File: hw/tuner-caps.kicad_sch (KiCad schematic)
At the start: 30 parts, among them K2101 G2RL-2, K2102 G2RL-2, K2103 G2RL-2, K2104 G2RL-2, K2105 G2RL-2, K2106 G2RL-2, K2107 G2RL-2, K2108 G2RL-2, K2109 G2RL-2, U2101 TPIC6C595PWR, U2102 TPIC6C595PWR

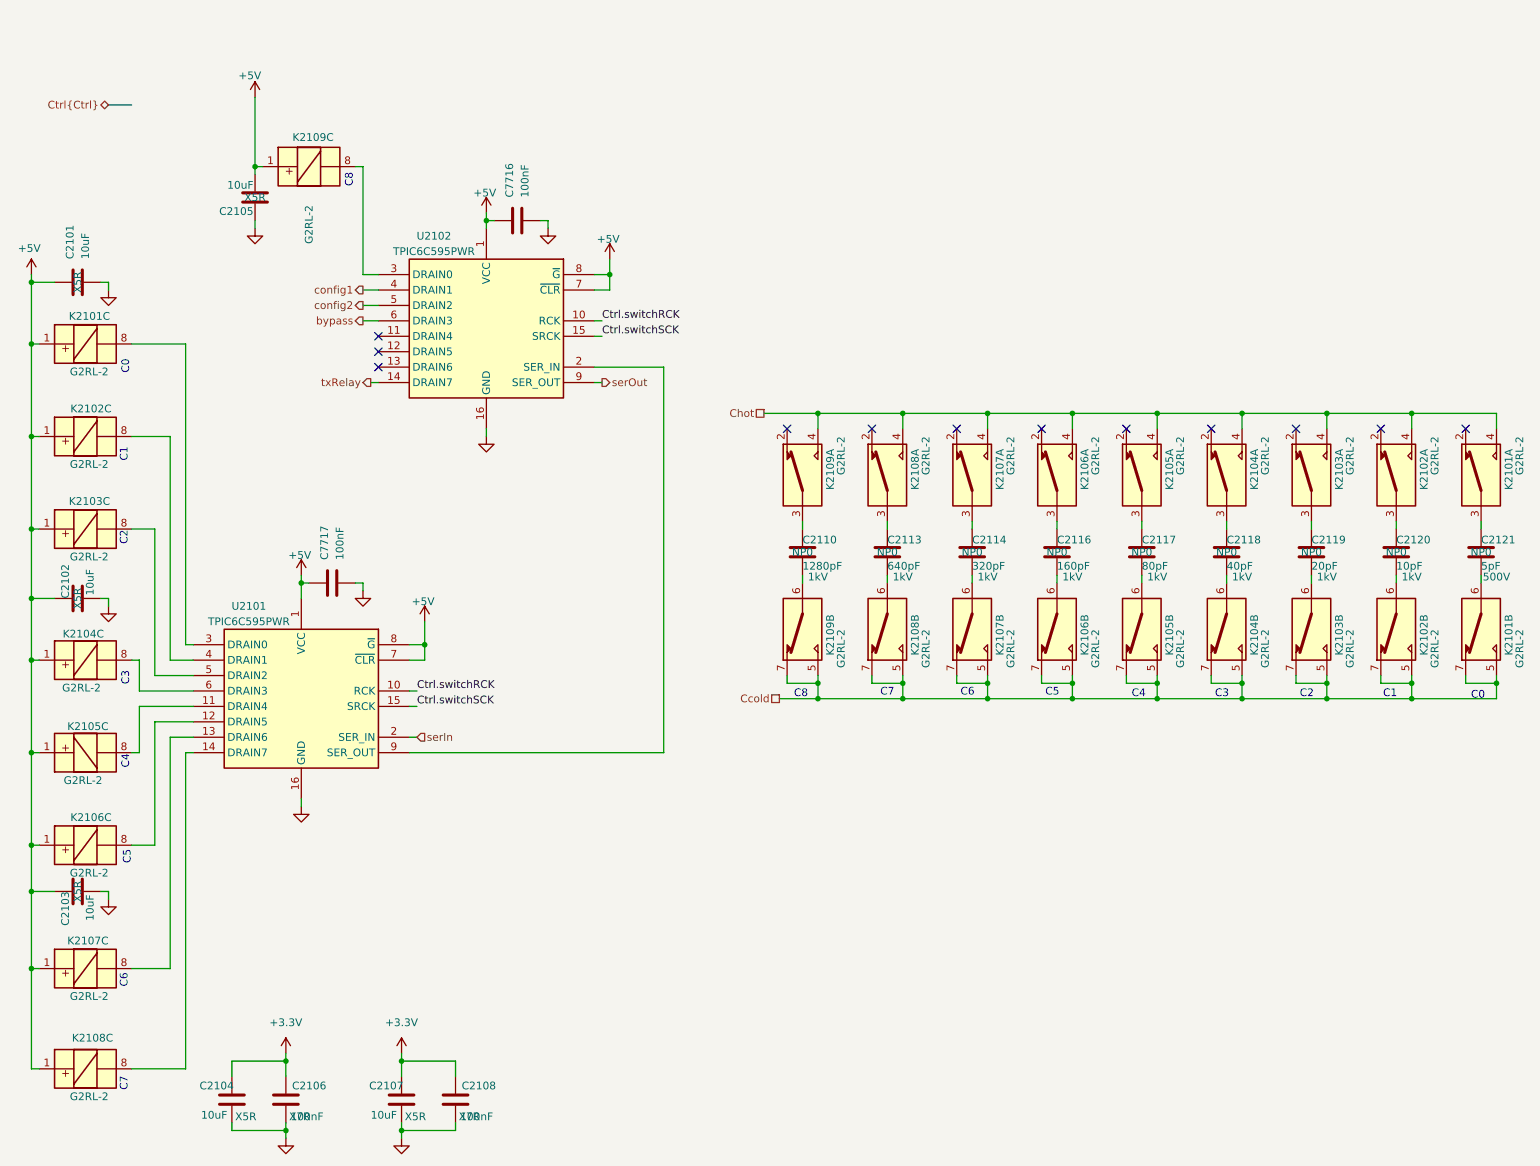
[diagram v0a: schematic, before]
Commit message: I think I have finished the relay conversion and 5V SPI I/O expander crap
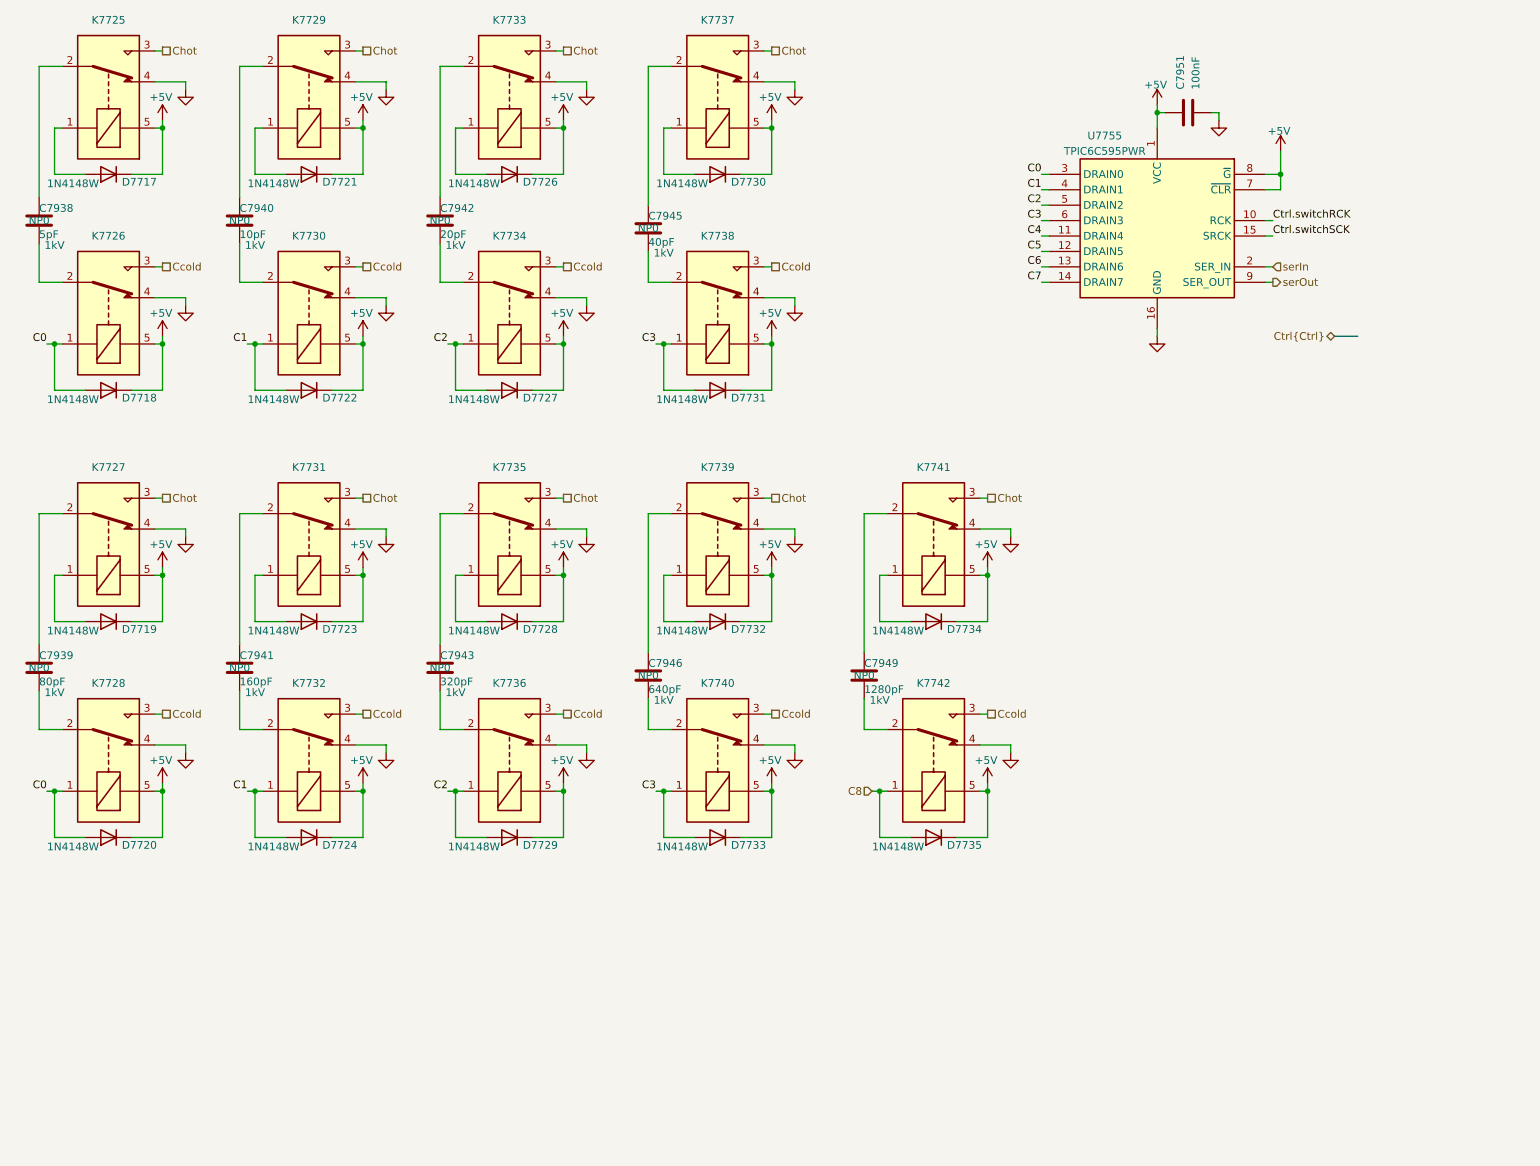
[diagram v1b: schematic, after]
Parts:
- removed C2101, C2102, C2103, C2104, C2105, C2107: 10uF, Capacitor_SMD:C_0805_2012Metric, symbol Device:C
- removed C2106, C2108: 100nF, Capacitor_SMD:C_0805_2012Metric, symbol Device:C
- removed C7716: 100nF, Capacitor_SMD:C_0603_1608Metric, symbol Device:C
- removed K2101, K2102, K2103, K2104, K2105, K2106, K2107, K2108, K2109: G2RL-2, Library:Relay_DPDT_Omron_G2RL-2, symbol Library:G2RL-2-functional
- removed U2102: TPIC6C595PWR, SOP65P640X120-16N, symbol Library:TPIC6C595PWR
- added D7717, D7718, D7719, D7720, D7721, D7722, D7723, D7724, D7726, D7727, D7728, D7729, D7730, D7731, D7732, D7733, D7734, D7735: 1N4148W, Diode_SMD:D_SOD-123, symbol Diode:1N4148W
- added K7725, K7726, K7727, K7728, K7729, K7730, K7731, K7732, K7733, K7734, K7735, K7736, K7737, K7738, K7739, K7740, K7741, K7742: G5Q-14-05, Relay_THT:Relay_SPDT_Omron-G5Q-1, symbol Relay:G5Q-1
- C7938: renamed from C2121; working-voltage 500V -> 1kV
- renumbered C2117 to C7939, C2120 to C7940, C2116 to C7941, C2119 to C7942, C2114 to C7943, C2118 to C7945, C2113 to C7946, C2110 to C7949, C7717 to C7951, U2101 to U7755
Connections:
- net +5V: now also D7717.1 (K), D7718.1 (K), D7719.1 (K), D7720.1 (K), D7721.1 (K), D7722.1 (K), D7723.1 (K), D7724.1 (K), D7726.1 (K), D7727.1 (K), D7728.1 (K), D7729.1 (K), D7730.1 (K), D7731.1 (K), D7732.1 (K), D7733.1 (K), D7734.1 (K), D7735.1 (K), K7725.5, K7726.5, K7727.5, K7728.5, K7729.5, K7730.5, K7731.5, K7732.5, K7733.5, K7734.5, K7735.5, K7736.5, K7737.5, K7738.5, K7739.5, K7740.5, K7741.5, K7742.5
- net Ccold: now also K7726.3, K7728.3, K7730.3, K7732.3, K7734.3, K7736.3, K7738.3, K7740.3, K7742.3
- net Chot: now also K7725.3, K7727.3, K7729.3, K7731.3, K7733.3, K7735.3, K7737.3, K7739.3, K7741.3
- net GND: now also K7725.4, K7726.4, K7727.4, K7728.4, K7729.4, K7730.4, K7731.4, K7732.4, K7733.4, K7734.4, K7735.4, K7736.4, K7737.4, K7738.4, K7739.4, K7740.4, K7741.4, K7742.4
- net serOut: now also U7755.9 (SER_OUT)
- net at C7949.1: now also K7741.2
- net at C7949.2: now also K7742.2
- net at C7942.1: now also K7733.2
- net at C7942.2: now also K7734.2
- net at C7941.1: now also K7731.2
- net at C7941.2: now also K7732.2
- net at C7943.1: now also K7735.2
- net at C7943.2: now also K7736.2
- net C1: now reaches U7755.4 (DRAIN1)
- net C1: now also D7722.2 (A), D7724.2 (A), K7730.1, K7732.1
- net at C7938.1: now also K7725.2
- net at C7938.2: now also K7726.2
- net at C7939.1: now also K7727.2
- net at C7939.2: now also K7728.2
- net C7: now reaches U7755.14 (DRAIN7)
- net C0: now reaches U7755.3 (DRAIN0)
- net C0: now also D7718.2 (A), D7720.2 (A), K7726.1, K7728.1
- net at C7946.1: now also K7739.2
- net at C7946.2: now also K7740.2
- net at C7940.2: now also K7730.2
- net at C7940.1: now also K7729.2
- net C6: now reaches U7755.13 (DRAIN6)
- net at C7945.1: now also K7737.2
- net at C7945.2: now also K7738.2
- net C5: now reaches U7755.12 (DRAIN5)
- net C4: now reaches U7755.11 (DRAIN4)
- net C2: now reaches U7755.5 (DRAIN2)
- net C2: now also D7727.2 (A), D7729.2 (A), K7734.1, K7736.1
- net C3: now reaches U7755.6 (DRAIN3)
- net C3: now also D7731.2 (A), D7733.2 (A), K7738.1, K7740.1
- new net: D7717.2 (A), K7725.1
- new net: D7719.2 (A), K7727.1
- new net: D7732.2 (A), K7739.1
- new net: D7730.2 (A), K7737.1
- new net: D7723.2 (A), K7731.1
- new net: D7721.2 (A), K7729.1
- new net: D7728.2 (A), K7735.1
- new net: D7726.2 (A), K7733.1
- new net: D7734.2 (A), K7741.1
- new net C8: D7735.2 (A), K7742.1
- no-connect marks 12 -> 0
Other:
- note removed: "C0"
- note removed: "C1"
- note removed: "C2"
- note removed: "C3"
- note removed: "C4"
- note removed: "C5"
- note removed: "C6"
- note removed: "C7"
- note removed: "C8"
- moved on the sheet: C7938, C7939, C7940, C7941, C7942, C7943, C7945, C7946, C7949, C7951, U7755
